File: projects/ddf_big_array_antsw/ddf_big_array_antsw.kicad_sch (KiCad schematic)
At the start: 75 parts, among them J1 Conn_Coaxial, J101 Conn_Coaxial, J102 Conn_Coaxial, J2 Conn_Coaxial, J201 Conn_Coaxial, J202 Conn_Coaxial, J3 Conn_Coaxial, J301 Conn_Coaxial, J302 Conn_Coaxial, J4 Conn_Coaxial, J401 Conn_Coaxial, J402 Conn_Coaxial, J5 Conn_Coaxial, J6 RJ45_Shielded, J7 RJ45_Shielded, J8 Conn_01x05_Male

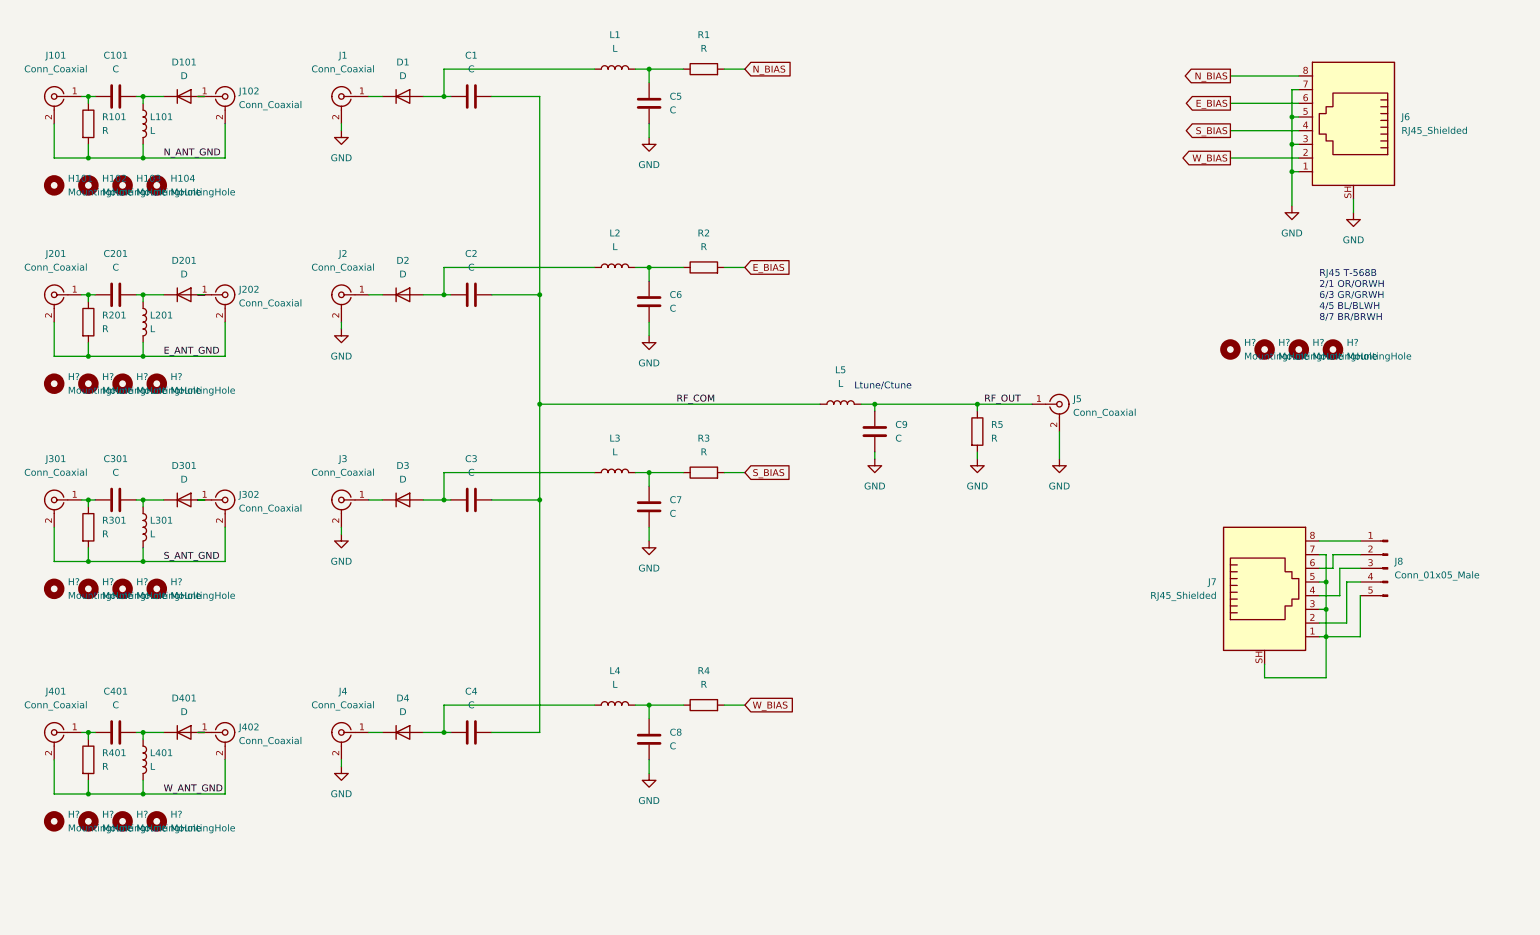
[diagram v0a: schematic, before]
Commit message: Checkpoint.
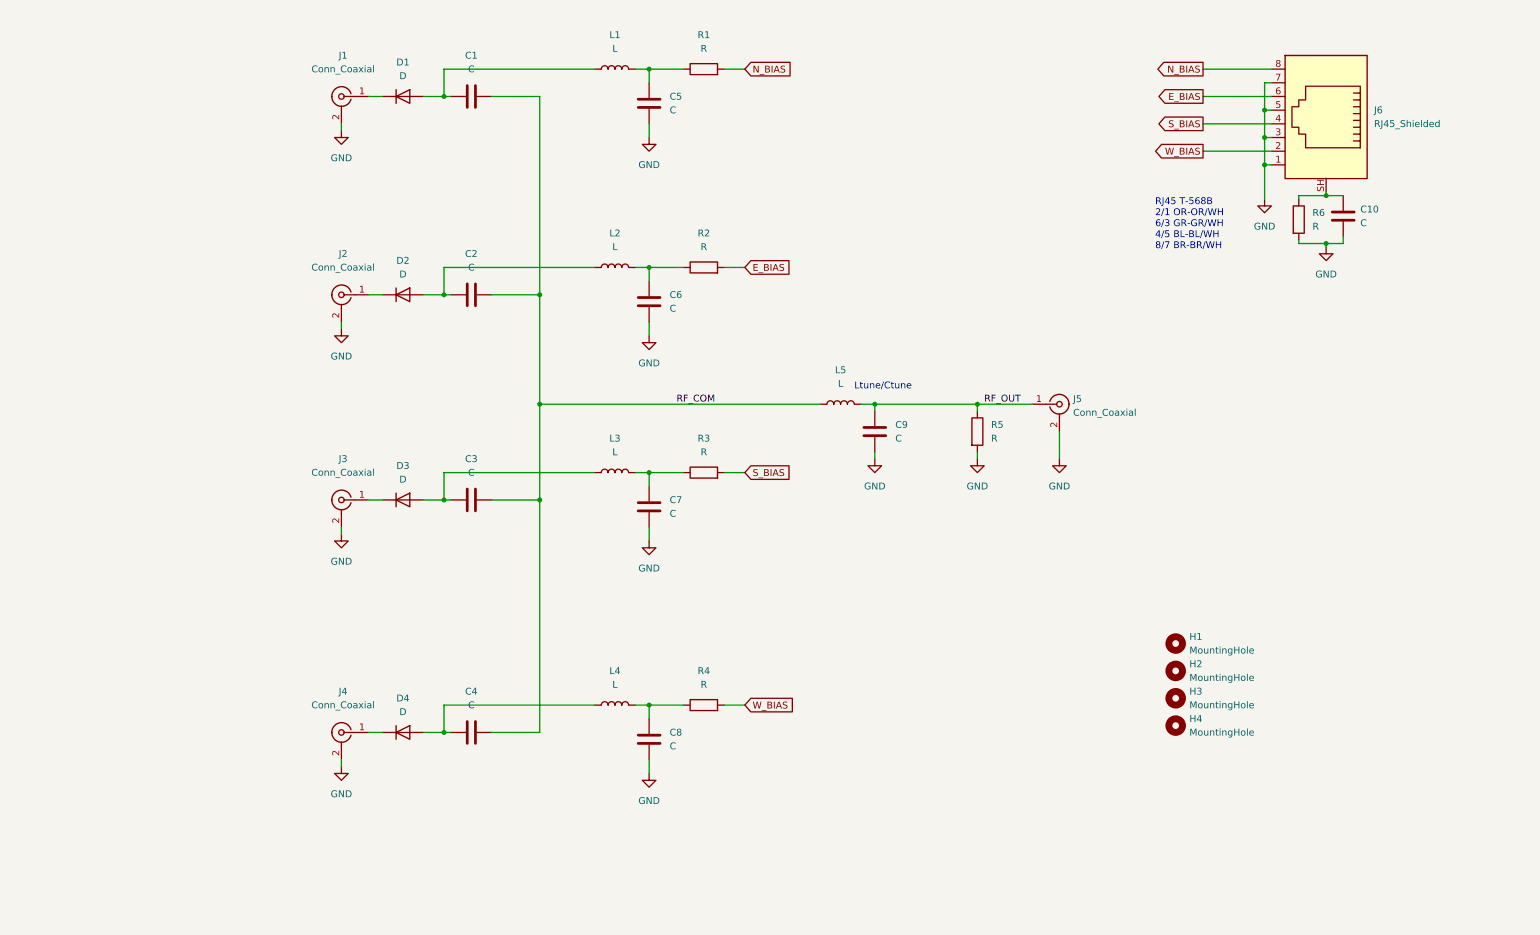
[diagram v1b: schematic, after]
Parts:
- removed C101, C201, C301, C401: C, Capacitor_SMD:C_0402_1005Metric_Pad0.74x0.62mm_HandSolder, symbol Device:C
- removed D101, D201, D301, D401: D, Diode_SMD:D_SOD-523, symbol Device:D
- removed H101, H102, H103, H104, H? (x12): MountingHole, symbol Mechanical:MountingHole
- removed J101, J201, J301, J401: Conn_Coaxial, Connector_Coaxial:SMA_Amphenol_132134_Vertical, symbol Connector:Conn_Coaxial
- removed J102, J202, J302, J402: Conn_Coaxial, Connector_Coaxial:SMA_Amphenol_132203-12_Horizontal, symbol Connector:Conn_Coaxial
- removed J7: RJ45_Shielded, Connector_RJ:RJ45_Wuerth_7499010001A_Horizontal, symbol Connector:RJ45_Shielded
- removed J8: Conn_01x05_Male, Connector_PinHeader_2.54mm:PinHeader_1x05_P2.54mm_Vertical, symbol Connector:Conn_01x05_Male
- removed L101, L201, L301, L401: L, Inductor_SMD:L_0402_1005Metric_Pad0.77x0.64mm_HandSolder, symbol Device:L
- removed R101, R201, R301, R401: R, Resistor_SMD:R_0402_1005Metric_Pad0.72x0.64mm_HandSolder, symbol Device:R
- added C10: C, Capacitor_SMD:C_0402_1005Metric_Pad0.74x0.62mm_HandSolder, symbol Device:C
- added R6: R, Resistor_SMD:R_0402_1005Metric_Pad0.72x0.64mm_HandSolder, symbol Device:R
- H1, H2, H3, H4: renamed from H?; footprint (none) -> MountingHole:MountingHole_3.2mm_M3
- J5: footprint Connector_Coaxial:SMA_Molex_73251-2200_Horizontal -> Connector_Coaxial:SMA_Amphenol_132203-12_Horizontal
- J6: footprint Connector_RJ:RJ45_Wuerth_7499010001A_Horizontal -> Connector_RJ:RJ45_Amphenol_RJHSE5380
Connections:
- net GND: now also C10.2, R6.2; no longer J6.SH
- new net: C10.1, J6.SH, R6.1
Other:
- note added: "RJ45 T-568B 2/1 OR-OR/WH 6/3 GR-GR/WH 4/5 BL-BL/WH 8/7 BR-BR/WH"
- note removed: "RJ45 T-568B 2/1 OR/ORWH 6/3 GR/GRWH 4/5 BL/BLWH 8/7 BR/BRWH"
- moved on the sheet: H1, H2, H3, H4, J6

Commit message: Checkpoint.
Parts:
- C10, C5, C6, C7, C8, C9: footprint Capacitor_SMD:C_0402_1005Metric_Pad0.74x0.62mm_HandSolder -> Capacitor_SMD:C_0603_1608Metric_Pad1.08x0.95mm_HandSolder
- R1, R2, R3, R4, R6: footprint Resistor_SMD:R_0402_1005Metric_Pad0.72x0.64mm_HandSolder -> Resistor_SMD:R_0603_1608Metric_Pad0.98x0.95mm_HandSolder
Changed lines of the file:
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@@
       (effects (font (size 1.27 1.27)) (justify left))
     )
-    (property "Footprint" "Capacitor_SMD:C_0402_1005Metric_Pad0.74x0.62mm_HandSolder" (id 2) (at 176.2252 101.6 0)
+    (property "Footprint" "Capacitor_SMD:C_0603_1608Metric_Pad1.08x0.95mm_HandSolder" (id 2) (at 176.2252 101.6 0)
       (effects (font (size 1.27 1.27)) hide)
     )
@@
     (property "Reference" "R3" (id 0) (at 143.51 99.06 90))
     (property "Value" "R" (id 1) (at 143.51 101.6 90))
-    (property "Footprint" "Resistor_SMD:R_0402_1005Metric_Pad0.72x0.64mm_HandSolder" (id 2) (at 143.51 107.188 90)
+    (property "Footprint" "Resistor_SMD:R_0603_1608Metric_Pad0.98x0.95mm_HandSolder" (id 2) (at 143.51 107.188 90)
       (effects (font (size 1.27 1.27)) hide)
     )
@@
       (effects (font (size 1.27 1.27)) (justify left))
     )
-    (property "Footprint" "Capacitor_SMD:C_0402_1005Metric_Pad0.74x0.62mm_HandSolder" (id 2) (at 263.2202 61.595 0)
+    (property "Footprint" "Capacitor_SMD:C_0603_1608Metric_Pad1.08x0.95mm_HandSolder" (id 2) (at 263.2202 61.595 0)
       (effects (font (size 1.27 1.27)) hide)
     )
@@
       (effects (font (size 1.27 1.27)) (justify left))
     )
-    (property "Footprint" "Capacitor_SMD:C_0402_1005Metric_Pad0.74x0.62mm_HandSolder" (id 2) (at 134.3152 158.75 0)
+    (property "Footprint" "Capacitor_SMD:C_0603_1608Metric_Pad1.08x0.95mm_HandSolder" (id 2) (at 134.3152 158.75 0)
       (effects (font (size 1.27 1.27)) hide)
     )
@@
     (property "Reference" "R1" (id 0) (at 143.51 24.13 90))
     (property "Value" "R" (id 1) (at 143.51 26.67 90))
-    (property "Footprint" "Resistor_SMD:R_0402_1005Metric_Pad0.72x0.64mm_HandSolder" (id 2) (at 143.51 32.258 90)
+    (property "Footprint" "Resistor_SMD:R_0603_1608Metric_Pad0.98x0.95mm_HandSolder" (id 2) (at 143.51 32.258 90)
       (effects (font (size 1.27 1.27)) hide)
     )
@@
     (property "Reference" "R2" (id 0) (at 143.51 60.96 90))
     (property "Value" "R" (id 1) (at 143.51 63.5 90))
-    (property "Footprint" "Resistor_SMD:R_0402_1005Metric_Pad0.72x0.64mm_HandSolder" (id 2) (at 143.51 69.088 90)
+    (property "Footprint" "Resistor_SMD:R_0603_1608Metric_Pad0.98x0.95mm_HandSolder" (id 2) (at 143.51 69.088 90)
       (effects (font (size 1.27 1.27)) hide)
     )
@@
       (effects (font (size 1.27 1.27)) (justify left))
     )
-    (property "Footprint" "Capacitor_SMD:C_0402_1005Metric_Pad0.74x0.62mm_HandSolder" (id 2) (at 134.3152 77.47 0)
+    (property "Footprint" "Capacitor_SMD:C_0603_1608Metric_Pad1.08x0.95mm_HandSolder" (id 2) (at 134.3152 77.47 0)
       (effects (font (size 1.27 1.27)) hide)
     )
@@
       (effects (font (size 1.27 1.27)) (justify left))
     )
-    (property "Footprint" "Resistor_SMD:R_0402_1005Metric_Pad0.72x0.64mm_HandSolder" (id 2) (at 252.222 58.42 90)
+    (property "Footprint" "Resistor_SMD:R_0603_1608Metric_Pad0.98x0.95mm_HandSolder" (id 2) (at 252.222 58.42 90)
       (effects (font (size 1.27 1.27)) hide)
     )
@@
       (effects (font (size 1.27 1.27)) (justify left))
     )
-    (property "Footprint" "Capacitor_SMD:C_0402_1005Metric_Pad0.74x0.62mm_HandSolder" (id 2) (at 134.3152 115.57 0)
+    (property "Footprint" "Capacitor_SMD:C_0603_1608Metric_Pad1.08x0.95mm_HandSolder" (id 2) (at 134.3152 115.57 0)
       (effects (font (size 1.27 1.27)) hide)
     )
@@
       (effects (font (size 1.27 1.27)) (justify left))
     )
-    (property "Footprint" "Capacitor_SMD:C_0402_1005Metric_Pad0.74x0.62mm_HandSolder" (id 2) (at 134.3152 40.64 0)
+    (property "Footprint" "Capacitor_SMD:C_0603_1608Metric_Pad1.08x0.95mm_HandSolder" (id 2) (at 134.3152 40.64 0)
       (effects (font (size 1.27 1.27)) hide)
     )
@@
     (property "Reference" "R4" (id 0) (at 143.51 142.24 90))
     (property "Value" "R" (id 1) (at 143.51 144.78 90))
-    (property "Footprint" "Resistor_SMD:R_0402_1005Metric_Pad0.72x0.64mm_HandSolder" (id 2) (at 143.51 150.368 90)
+    (property "Footprint" "Resistor_SMD:R_0603_1608Metric_Pad0.98x0.95mm_HandSolder" (id 2) (at 143.51 150.368 90)
       (effects (font (size 1.27 1.27)) hide)
     )
@@
     )
     (path "/ebee6295-95a0-4b78-820c-724e9fe8bc5d"
-      (reference "C5") (unit 1) (value "C") (footprint "Capacitor_SMD:C_0402_1005Metric_Pad0.74x0.62mm_HandSolder")
+      (reference "C5") (unit 1) (value "C") (footprint "Capacitor_SMD:C_0603_1608Metric_Pad1.08x0.95mm_HandSolder")
     )
     (path "/b70c6f80-9f0b-49ff-9760-23326927c8f4"
-      (reference "C6") (unit 1) (value "C") (footprint "Capacitor_SMD:C_0402_1005Metric_Pad0.74x0.62mm_HandSolder")
+      (reference "C6") (unit 1) (value "C") (footprint "Capacitor_SMD:C_0603_1608Metric_Pad1.08x0.95mm_HandSolder")
     )
     (path "/ea6d3061-13c4-4746-914e-a9591b4c7d84"
-      (reference "C7") (unit 1) (value "C") (footprint "Capacitor_SMD:C_0402_1005Metric_Pad0.74x0.62mm_HandSolder")
+      (reference "C7") (unit 1) (value "C") (footprint "Capacitor_SMD:C_0603_1608Metric_Pad1.08x0.95mm_HandSolder")
     )
     (path "/3e60d1a2-bbc3-478a-bd1a-757741907e9c"
-      (reference "C8") (unit 1) (value "C") (footprint "Capacitor_SMD:C_0402_1005Metric_Pad0.74x0.62mm_HandSolder")
+      (reference "C8") (unit 1) (value "C") (footprint "Capacitor_SMD:C_0603_1608Metric_Pad1.08x0.95mm_HandSolder")
     )
     (path "/11144e59-10a0-41f7-a9d6-bbbd2d208879"
-      (reference "C9") (unit 1) (value "C") (footprint "Capacitor_SMD:C_0402_1005Metric_Pad0.74x0.62mm_HandSolder")
+      (reference "C9") (unit 1) (value "C") (footprint "Capacitor_SMD:C_0603_1608Metric_Pad1.08x0.95mm_HandSolder")
     )
     (path "/2ba52fdd-6a8d-41ac-bb4a-7a0252982099"
-      (reference "C10") (unit 1) (value "C") (footprint "Capacitor_SMD:C_0402_1005Metric_Pad0.74x0.62mm_HandSolder")
+      (reference "C10") (unit 1) (value "C") (footprint "Capacitor_SMD:C_0603_1608Metric_Pad1.08x0.95mm_HandSolder")
     )
     (path "/57fb8ada-7623-4a7f-90a6-450a79e03e45"
@@
     )
     (path "/57956bab-b0fc-4027-bfc7-29ac34f67c29"
-      (reference "R1") (unit 1) (value "R") (footprint "Resistor_SMD:R_0402_1005Metric_Pad0.72x0.64mm_HandSolder")
+      (reference "R1") (unit 1) (value "R") (footprint "Resistor_SMD:R_0603_1608Metric_Pad0.98x0.95mm_HandSolder")
     )
     (path "/972d5e10-1a1c-4b23-a90f-f4f171587b05"
-      (reference "R2") (unit 1) (value "R") (footprint "Resistor_SMD:R_0402_1005Metric_Pad0.72x0.64mm_HandSolder")
+      (reference "R2") (unit 1) (value "R") (footprint "Resistor_SMD:R_0603_1608Metric_Pad0.98x0.95mm_HandSolder")
     )
     (path "/24cc2e59-0230-478d-b9ef-ad89fb1b17c0"
-      (reference "R3") (unit 1) (value "R") (footprint "Resistor_SMD:R_0402_1005Metric_Pad0.72x0.64mm_HandSolder")
+      (reference "R3") (unit 1) (value "R") (footprint "Resistor_SMD:R_0603_1608Metric_Pad0.98x0.95mm_HandSolder")
     )
     (path "/fdad155e-2f66-4e23-8c55-b0a7057b87ce"
-      (reference "R4") (unit 1) (value "R") (footprint "Resistor_SMD:R_0402_1005Metric_Pad0.72x0.64mm_HandSolder")
+      (reference "R4") (unit 1) (value "R") (footprint "Resistor_SMD:R_0603_1608Metric_Pad0.98x0.95mm_HandSolder")
     )
     (path "/0d7b6121-7f90-44b2-bdc3-d3f8e3779c1e"
@@
     )
     (path "/bae019c3-57d4-4c72-832f-fab263ff9cca"
-      (reference "R6") (unit 1) (value "R") (footprint "Resistor_SMD:R_0402_1005Metric_Pad0.72x0.64mm_HandSolder")
-    )
-  )
+      (reference "R6") (unit 1) (value "R") (footprint "Resistor_SMD:R_0603_1608Metric_Pad0.98x0.95mm_HandSolder")
+    )
+  )
